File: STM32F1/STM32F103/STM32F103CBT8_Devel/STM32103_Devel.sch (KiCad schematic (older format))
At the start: 46 parts, among them J1 Conn_02x03_Odd_Even, J2 USB_B_Micro, J3 Conn_02x10_Odd_Even, J4 Conn_01x16, J5 Conn_01x16, J6 Conn_02x05 Odd_Even, SW1 SW_Push, U1 STM32F103CBTx, U2 AMS1117-3.3, Y1 8MHz, Y2 Crystal

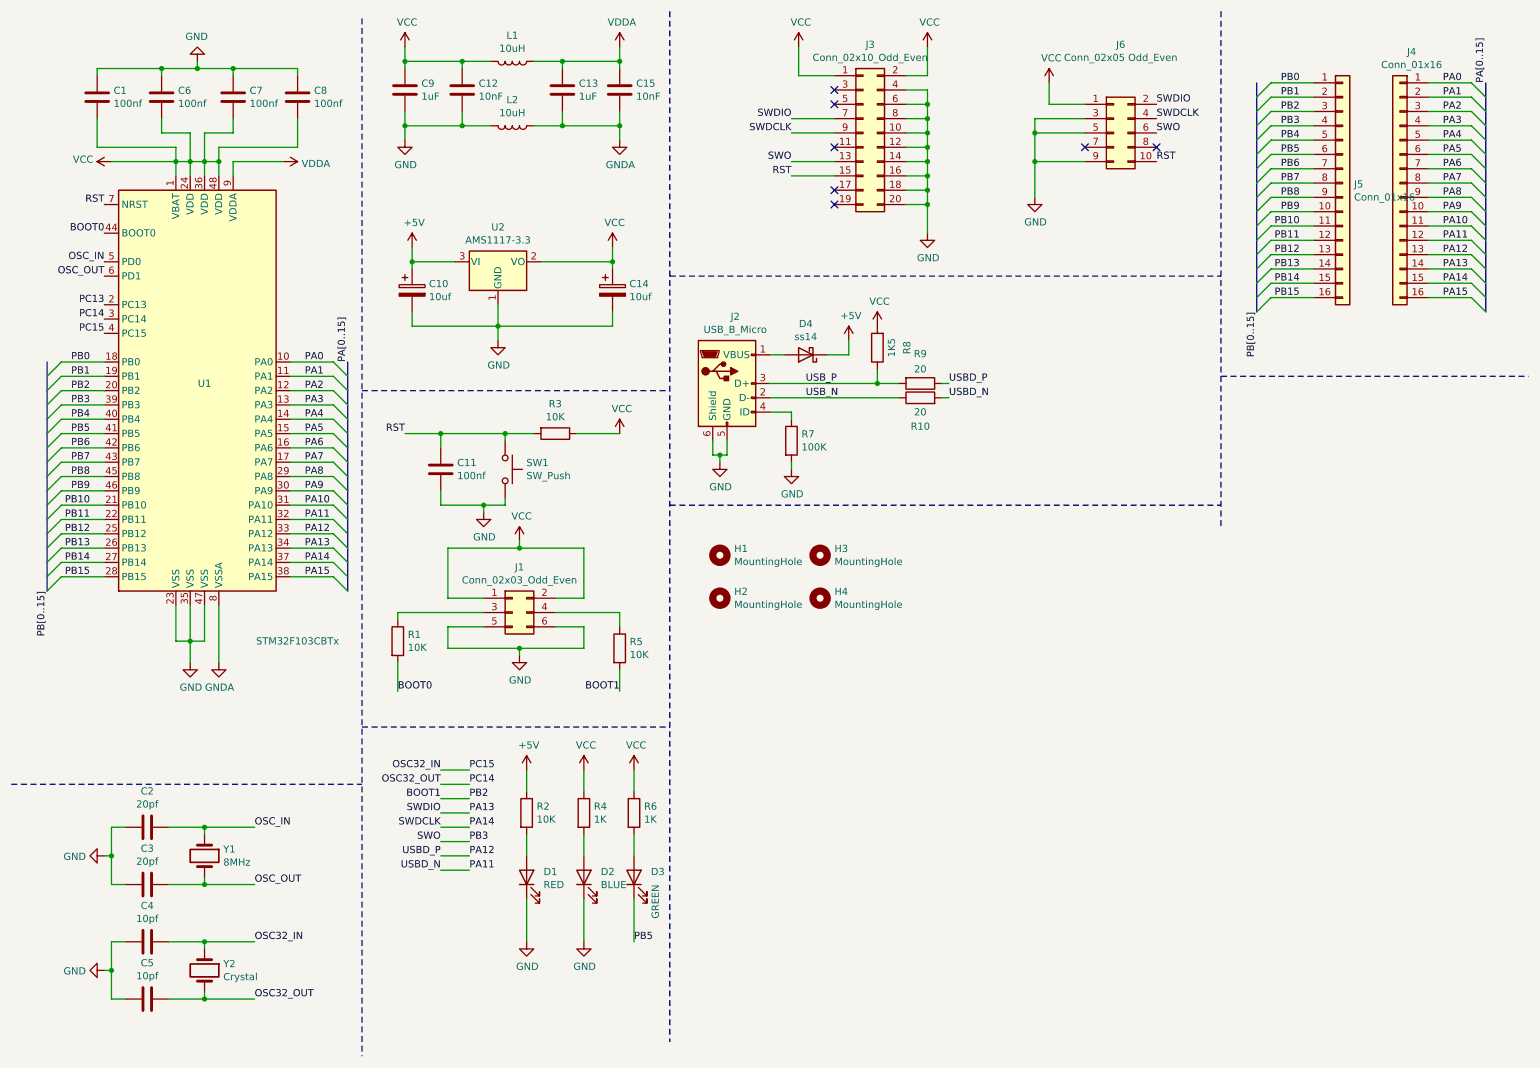
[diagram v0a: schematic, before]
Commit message: Kicad Reorg
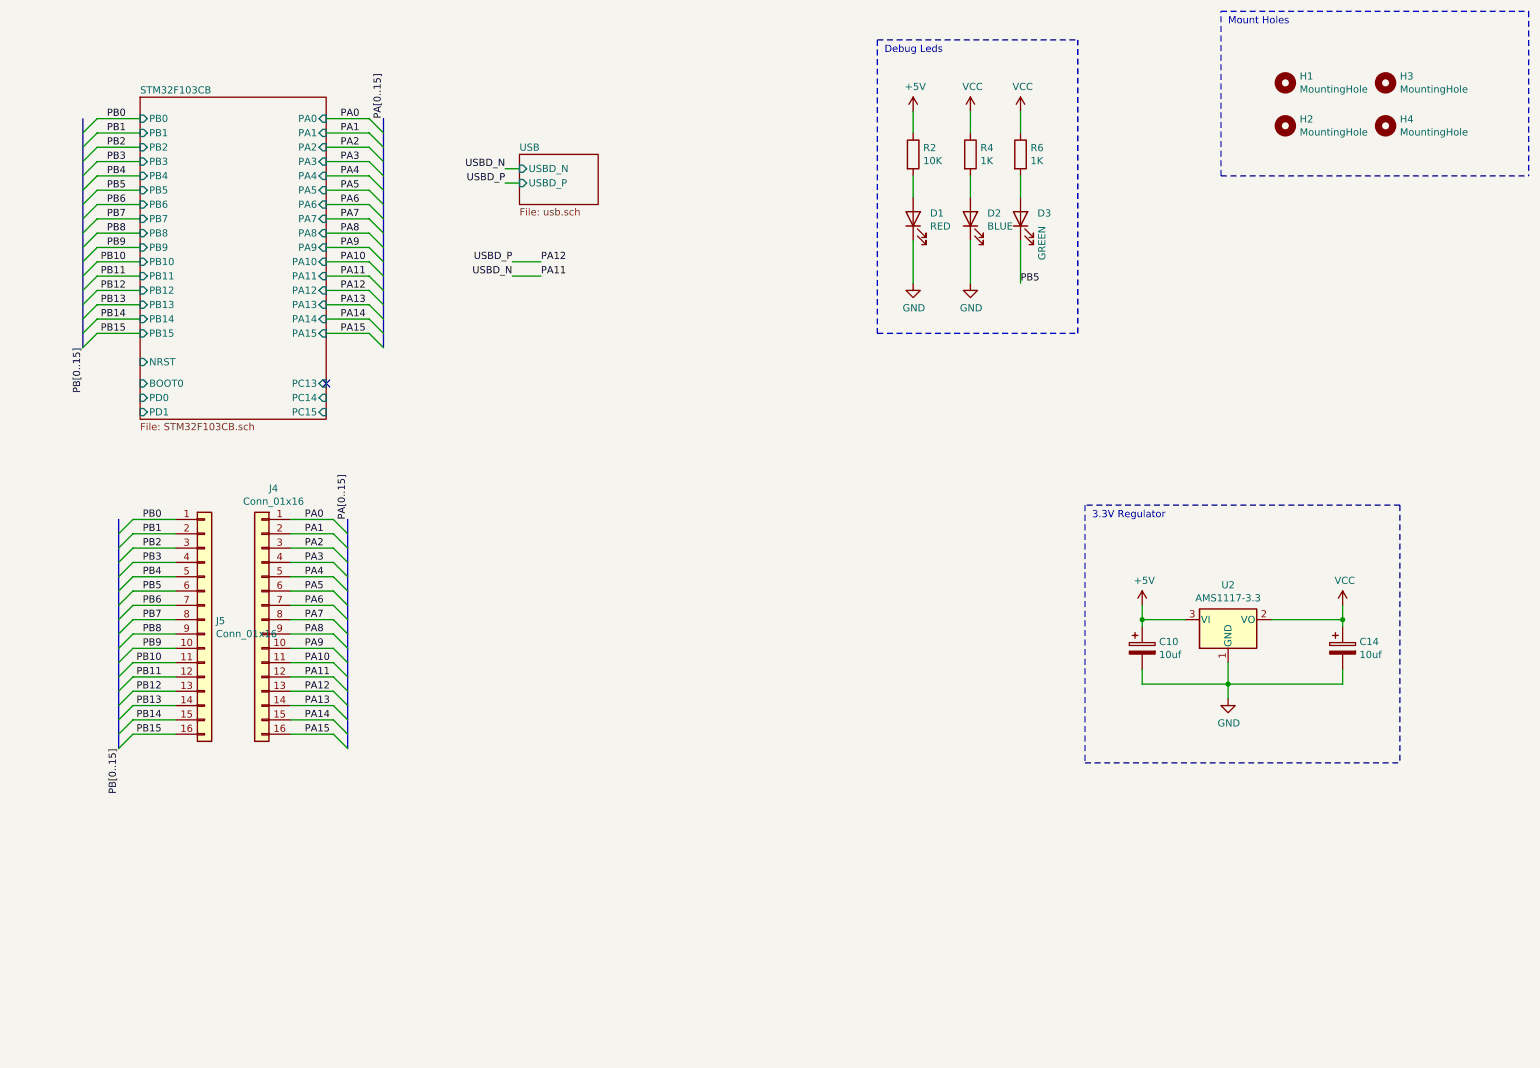
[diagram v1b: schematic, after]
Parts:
- removed C1, C11, C6, C7, C8: 100nf, Capacitor_SMD:C_0805_2012Metric, symbol Device:C
- removed C12, C15: 10nF, Capacitor_SMD:C_0805_2012Metric, symbol Device:C
- removed C13, C9: 1uF, Capacitor_SMD:C_0805_2012Metric, symbol Device:C
- removed C2, C3: 20pf, Capacitor_SMD:C_0805_2012Metric, symbol Device:C
- removed C4, C5: 10pf, Capacitor_SMD:C_0805_2012Metric, symbol Device:C
- removed D4: ss14, Diode_SMD:D_SMA, symbol Device:D_Schottky
- removed J1: Conn_02x03_Odd_Even, Connector_PinHeader_2.54mm:PinHeader_2x03_P2.54mm_Vertical, symbol Connector_Generic:Conn_02x03_Odd_Even
- removed J2: USB_B_Micro, Connector_USB:USB_Micro-B_Wuerth_629105150521_CircularHoles, symbol STM32103_Devel-rescue:USB_B_Micro-Connector
- removed J3: Conn_02x10_Odd_Even, Connector_PinHeader_2.54mm:PinHeader_2x10_P2.54mm_Vertical, symbol Connector_Generic:Conn_02x10_Odd_Even
- removed J6: Conn_02x05 Odd_Even, Connector_PinHeader_1.27mm:PinHeader_2x05_P1.27mm_Vertical, symbol Connector_Generic:Conn_02x05_Odd_Even
- removed L1, L2: 10uH, Inductor_SMD:L_0805_2012Metric, symbol Device:L
- removed R1, R3, R5: 10K, Resistor_SMD:R_0805_2012Metric, symbol Device:R
- removed R10, R9: 20, Resistor_SMD:R_0805_2012Metric, symbol Device:R
- removed R7: 100K, Resistor_SMD:R_0805_2012Metric, symbol Device:R
- removed R8: 1K5, Resistor_SMD:R_0805_2012Metric, symbol Device:R
- removed SW1: SW_Push, Button_Switch_THT:SW_PUSH_6mm, symbol Switch:SW_Push
- removed U1: STM32F103CBTx, STM32103_Devel:LQFP-48_7x7mm_P0.5mm, symbol MCU_ST_STM32F1:STM32F103CBTx
- removed Y1: 8MHz, Crystal:Crystal_SMD_5032-2Pin_5.0x3.2mm, symbol Device:Crystal
- removed Y2: Crystal, Crystal:Crystal_SMD_3215-2Pin_3.2x1.5mm, symbol Device:Crystal
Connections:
- net BOOT1 renamed PB2
- no-connect marks 7 -> 1
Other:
- note added: "3.3V Regulator"
- note added: "Debug Leds"
- note added: "Mount Holes"
- moved on the sheet: C10, C14, D1, D2, D3, H1, H2, H3, H4, J4, J5, R2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
